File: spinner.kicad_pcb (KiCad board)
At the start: 2 copper layers, 147 x 147 mm, 134 parts, among them J1 Micro_SD_Card, J301 USB_C_Receptacle_USB2.0_16P, SW1 SW_SPDT, SW301 RESET, SW302 BOOT, U2 RS0102, U301 BQ24073RGT, U302 SPX3819M5-L-3-3, U303 TPS61022, u10 ESP32-S3-WROOM-1

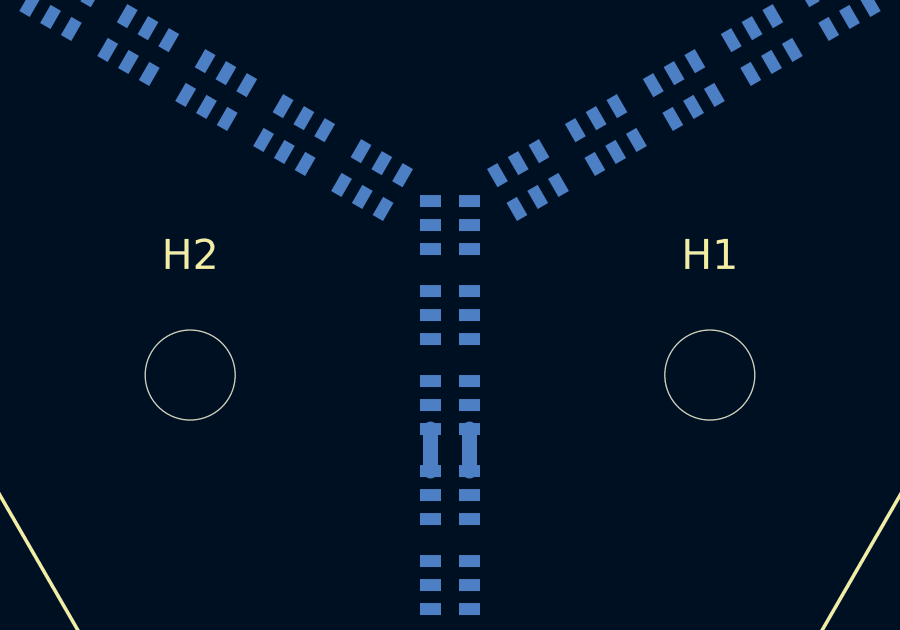
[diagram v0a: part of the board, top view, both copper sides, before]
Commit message: IDK.  Some routing.
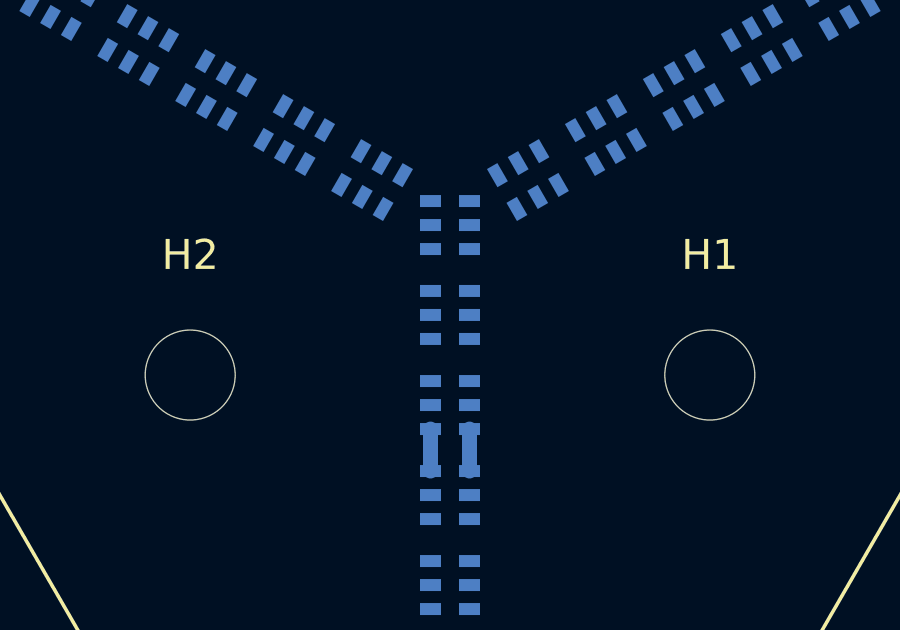
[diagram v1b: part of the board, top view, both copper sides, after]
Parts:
- moved D101 3.00 mm to (150.0, 100.0)
- moved D0 3.00 mm to (150.0, 103.0)
- renumbered D101 to D0, D0 to D101
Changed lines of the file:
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@@
 	(footprint "Library:SK9822-hakz"
 		(layer "B.Cu")
-		(at 150 103)
+		(at 150 100)
 		(descr "http://www.led-color.com/upload/201604/APA102-2020%20SMD%20LED.pdf")
 		(tags "LED RGB SPI")
-		(property "Reference" "D0"
+		(property "Reference" "D101"
 			(at 0 -2.11 0)
 			(layer "B.SilkS")
@@
 	(footprint "Library:SK9822-hakz"
 		(layer "B.Cu")
-		(at 150 100)
+		(at 150 102.9972)
 		(descr "http://www.led-color.com/upload/201604/APA102-2020%20SMD%20LED.pdf")
 		(tags "LED RGB SPI")
-		(property "Reference" "D101"
+		(property "Reference" "D0"
 			(at 0 -2.11 0)
 			(layer "B.SilkS")
